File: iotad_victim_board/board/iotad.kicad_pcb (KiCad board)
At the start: 2 copper layers, 24.8 x 29 mm, 5 parts, among them P1 CONN_01X09, P2 CONN_01X06, U1 24C16, U2 MAX31820

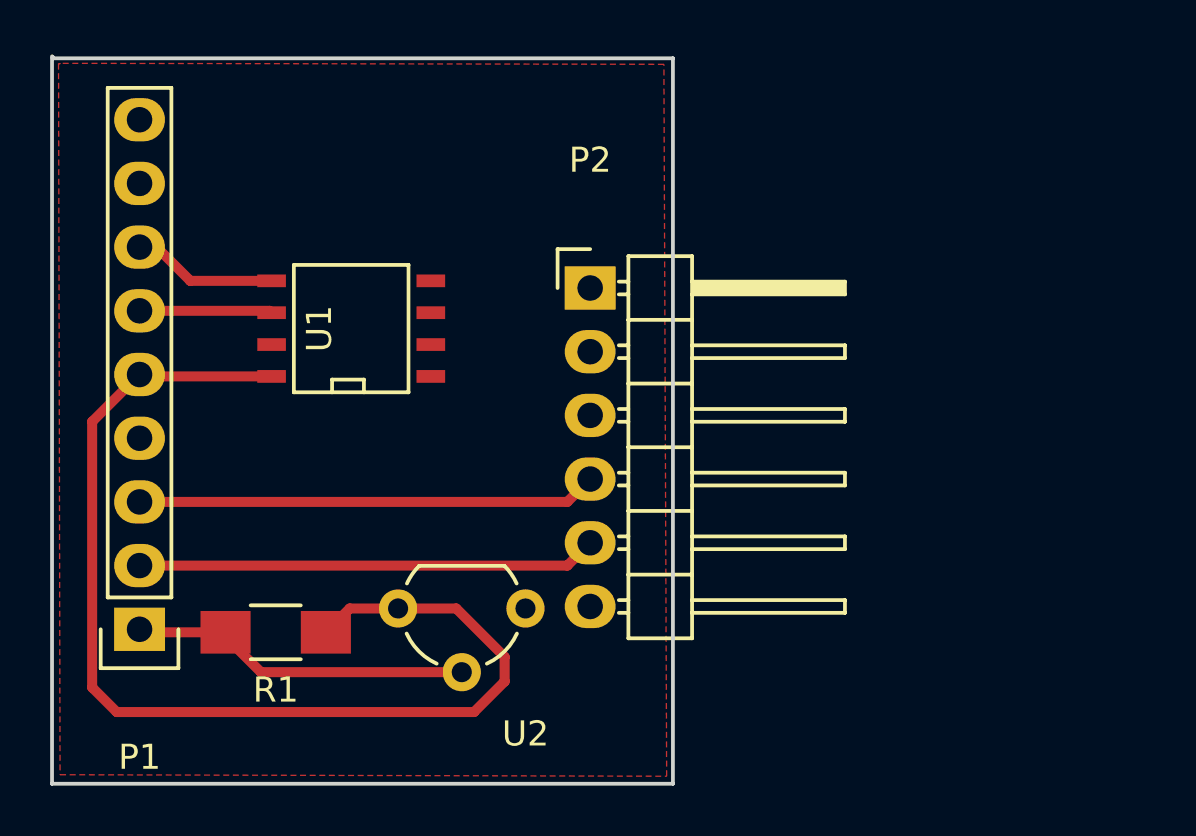
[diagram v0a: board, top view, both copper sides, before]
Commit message: today
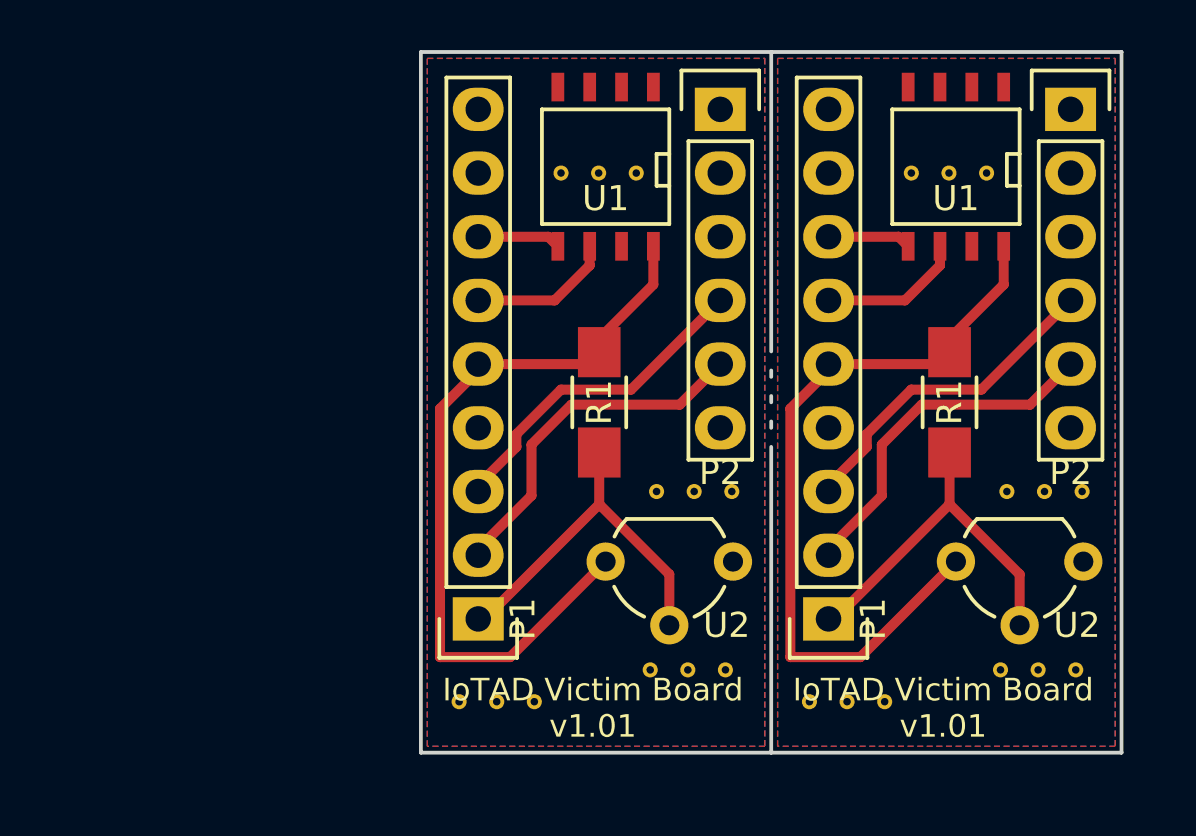
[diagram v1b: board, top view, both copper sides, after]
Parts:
- removed the P1 at (125.9, 124.6)
- removed the P2 at (143.9, 111.0)
- removed the R1 at (131.4, 124.7)
- removed the U1 at (134.4, 112.6)
- removed the U2 at (141.3, 123.8)
- added P1: CONN_01X09, Pin_Headers:Pin_Header_Straight_1x09, F.Cu at (153.4, 124.2)
- added P1: CONN_01X09, Pin_Headers:Pin_Header_Straight_1x09, F.Cu at (139.4, 124.2)
- added P2: CONN_01X06, Pin_Headers:Pin_Header_Straight_1x06, F.Cu at (163.1, 103.9)
- added P2: CONN_01X06, Pin_Headers:Pin_Header_Straight_1x06, F.Cu at (149.1, 103.9)
- added R1: 4.8k, Resistors_SMD:R_1206_HandSoldering, F.Cu at (158.2, 115.6)
- added R1: 4.8k, Resistors_SMD:R_1206_HandSoldering, F.Cu at (144.3, 115.6)
- added REF**11111: via, via, F.Cu at (152.7, 127.5)
- added REF**11111: via, via, F.Cu at (160.3, 126.2)
- added REF**11111: via, via, F.Cu at (160.5, 119.1)
- added REF**11111: via, via, F.Cu at (156.7, 106.4)
- added REF**11111: via, via, F.Cu at (146.3, 126.2)
- added REF**11111: via, via, F.Cu at (138.7, 127.5)
- added REF**11111: via, via, F.Cu at (146.6, 119.1)
- added REF**11111: via, via, F.Cu at (142.7, 106.4)
- added REF**11121: via, via, F.Cu at (161.8, 126.2)
- added REF**11121: via, via, F.Cu at (154.2, 127.5)
- added REF**11121: via, via, F.Cu at (162.0, 119.1)
- added REF**11121: via, via, F.Cu at (158.2, 106.4)
- added REF**11121: via, via, F.Cu at (147.8, 126.2)
- added REF**11121: via, via, F.Cu at (140.2, 127.5)
- added REF**11121: via, via, F.Cu at (148.1, 119.1)
- added REF**11121: via, via, F.Cu at (144.2, 106.4)
- added REF**11131: via, via, F.Cu at (155.7, 127.5)
- added REF**11131: via, via, F.Cu at (163.5, 119.1)
- added REF**11131: via, via, F.Cu at (163.3, 126.2)
- added REF**11131: via, via, F.Cu at (159.7, 106.4)
- added REF**11131: via, via, F.Cu at (149.3, 126.2)
- added REF**11131: via, via, F.Cu at (141.7, 127.5)
- added REF**11131: via, via, F.Cu at (149.6, 119.1)
- added REF**11131: via, via, F.Cu at (145.7, 106.4)
- added U1: 24C16, SMD_Packages:SOIC-8-N, F.Cu at (158.5, 106.2)
- added U1: 24C16, SMD_Packages:SOIC-8-N, F.Cu at (144.5, 106.2)
- added U2: MAX31820, TO_SOT_Packages_THT:TO-92_Molded_Wide, F.Cu at (163.6, 121.9)
- added U2: MAX31820, TO_SOT_Packages_THT:TO-92_Molded_Wide, F.Cu at (149.6, 121.9)
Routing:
- net VCC: track 45.2 -> 61.2 mm
- net DATA: track 13.7 -> 29.5 mm
- net TX: track 18.3 -> 28.3 mm
- net RX: track 18.3 -> 26.5 mm
- net SCL: track 5.30 -> 11.6 mm
- net SDA: track 5.82 -> 6.67 mm
- added copper zone on B.Cu, net Net-(P1-Pad8)
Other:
- board size 24.8 x 29 mm -> 27.9 x 27.9 mm
- board text added: "3.3v"
- board text added: "D1W"
- board text added: "GND"
- board text added: "IoTAD Victim Board v1.01"
- board text added: "RX"
- board text added: "SCL"
- board text added: "SDA"
- board text added: "TX"
- board text added: "dsgn: jegeva 2016"
